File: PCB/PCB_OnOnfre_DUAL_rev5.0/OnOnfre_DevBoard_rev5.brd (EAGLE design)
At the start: 44 x 43.9 mm, 30 parts, among them J3Y S8050, J7 8p, K1 OMRON-G3MB-202P-SSR2, K2 OMRON-G3MB-202P-SSR2, U2 esp12

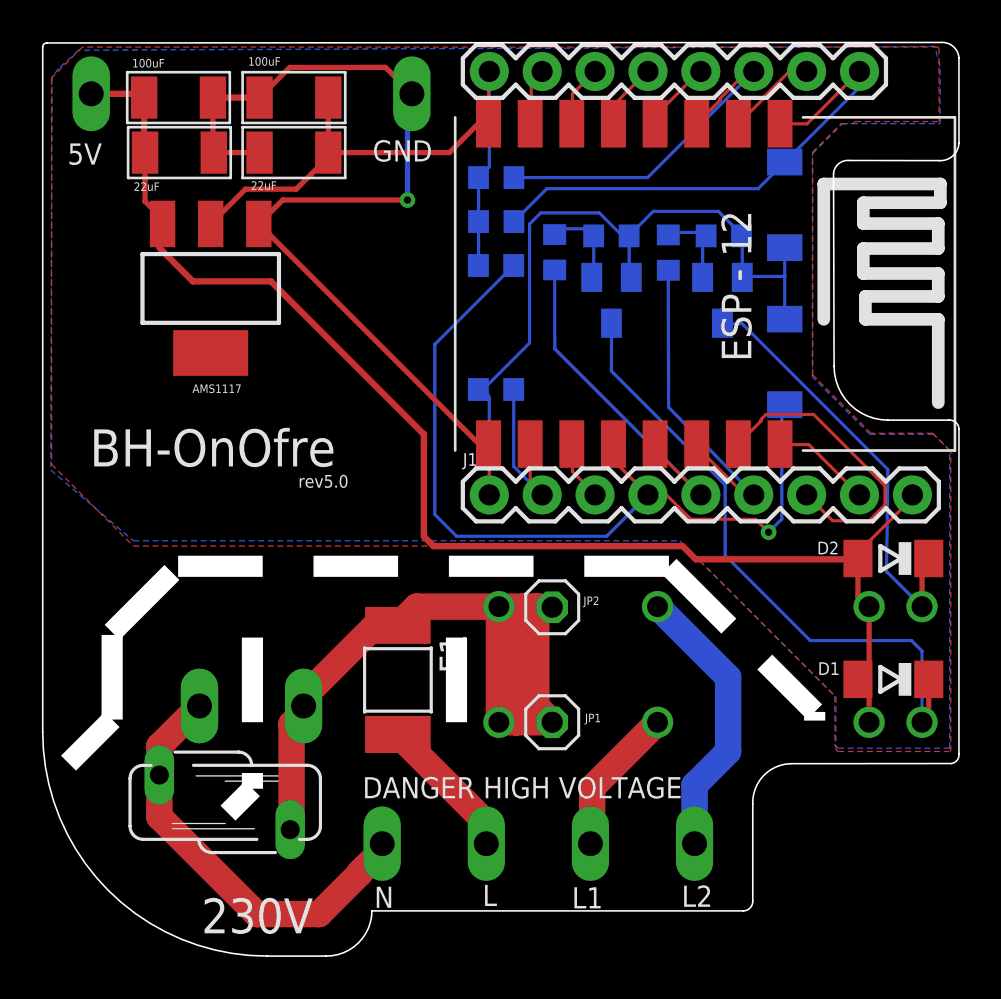
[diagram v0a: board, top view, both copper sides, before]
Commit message: rev5
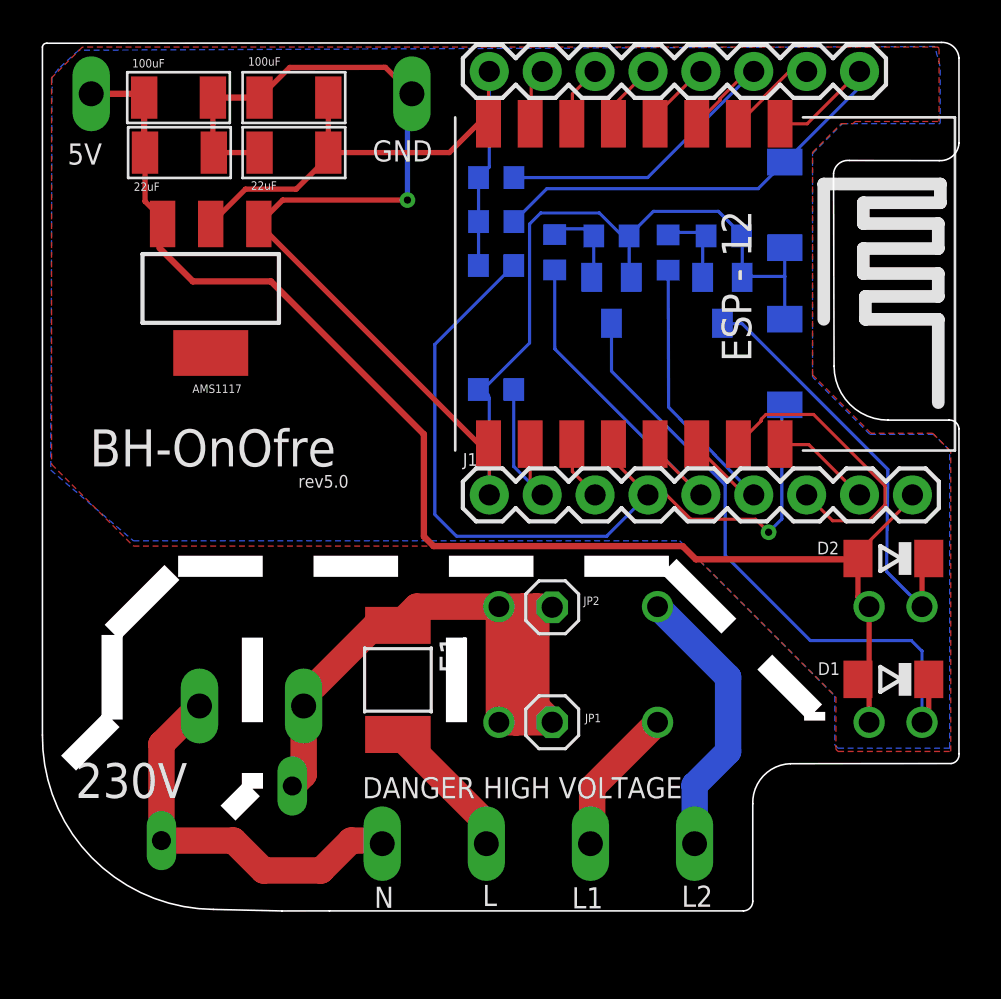
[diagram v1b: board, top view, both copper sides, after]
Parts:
- moved R5 0.54 mm to (9.56, 9.35), flipped to the bottom, turned to 270 degrees
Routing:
- net LINE_L: track 40.0 -> 37.7 mm
- net NEUTRAL_IN: track 20.1 -> 19.1 mm
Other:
- board size 44 x 43.9 mm -> 44 x 41.7 mm
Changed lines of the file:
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@@
 <grid distance="0.000123031496" unitdist="mil" unit="mil" style="lines" multiple="1" display="yes" altdistance="5" altunitdist="mil" altunit="mil"/>
 <layers>
-<layer number="1" name="Top" color="4" fill="1" visible="no" active="yes"/>
+<layer number="1" name="Top" color="4" fill="1" visible="yes" active="yes"/>
 <layer number="2" name="Route2" color="1" fill="3" visible="no" active="no"/>
 <layer number="3" name="Route3" color="4" fill="3" visible="no" active="no"/>
@@
 <layer number="25" name="tNames" color="7" fill="1" visible="yes" active="yes"/>
 <layer number="26" name="bNames" color="7" fill="1" visible="yes" active="yes"/>
-<layer number="27" name="tValues" color="7" fill="1" visible="yes" active="yes"/>
-<layer number="28" name="bValues" color="7" fill="1" visible="yes" active="yes"/>
+<layer number="27" name="tValues" color="7" fill="1" visible="no" active="yes"/>
+<layer number="28" name="bValues" color="7" fill="1" visible="no" active="yes"/>
 <layer number="29" name="tStop" color="7" fill="3" visible="no" active="yes"/>
 <layer number="30" name="bStop" color="7" fill="6" visible="no" active="yes"/>
@@
 <layer number="42" name="bRestrict" color="1" fill="10" visible="yes" active="yes"/>
 <layer number="43" name="vRestrict" color="2" fill="10" visible="no" active="yes"/>
-<layer number="44" name="Drills" color="7" fill="1" visible="yes" active="yes"/>
-<layer number="45" name="Holes" color="7" fill="1" visible="yes" active="yes"/>
-<layer number="46" name="Milling" color="3" fill="1" visible="yes" active="yes"/>
+<layer number="44" name="Drills" color="7" fill="1" visible="no" active="yes"/>
+<layer number="45" name="Holes" color="7" fill="1" visible="no" active="yes"/>
+<layer number="46" name="Milling" color="3" fill="1" visible="no" active="yes"/>
 <layer number="47" name="Measures" color="7" fill="1" visible="no" active="yes"/>
 <layer number="48" name="Document" color="7" fill="1" visible="no" active="yes"/>
@@
 <text x="33.608865625" y="25.98010625" size="0.6096" layer="26" font="vector" ratio="13" rot="MR45">L1</text>
 <text x="36.1006125" y="26.021965625" size="0.6096" layer="26" font="vector" ratio="13" rot="MR45">L2</text>
-<text x="8.320915625" y="3.579975" size="1.6764" layer="25" font="vector" ratio="13">230V</text>
+<text x="2.2720875" y="10.07901875" size="1.6764" layer="25" font="vector" ratio="13">230V</text>
 <text x="27.607209375" y="5.793196875" size="1.016" layer="25" font="vector" ratio="13" rot="R180">L1</text>
 <text x="12.972021875" y="24.981884375" size="0.6096" layer="25">rev5.0</text>
 <text x="12.192" y="12.446" size="0.4064" layer="26" rot="MR0">HLK-PM01</text>
-<wire x1="0.6984" y1="46.1592125" x2="0.6984" y2="13.243003125" width="0.0762" layer="20"/>
-<wire x1="0.6984" y1="13.243003125" x2="11.463928125" y2="2.487625" width="0.0762" layer="20" curve="90"/>
-<wire x1="11.463928125" y1="2.487625" x2="14.302721875" y2="2.487625" width="0.0762" layer="20"/>
-<wire x1="14.302721875" y1="2.487625" x2="16.511228125" y2="4.65789375" width="0.0762" layer="20" curve="90"/>
-<wire x1="16.511228125" y1="4.65789375" x2="34.35341875" y2="4.65789375" width="0.0762" layer="20"/>
+<wire x1="0.68574375" y1="46.14655625" x2="0.68574375" y2="13.103775" width="0.0762" layer="20"/>
+<wire x1="0.68574375" y1="13.103775" x2="8.892471875" y2="4.72859375" width="0.0762" layer="20" curve="90"/>
+<wire x1="8.892471875" y1="4.72859375" x2="12.19380625" y2="4.654959375" width="0.0762" layer="20"/>
+<wire x1="12.19380625" y1="4.654959375" x2="14.468953125" y2="4.657896875" width="0.0762" layer="20"/>
+<wire x1="14.468953125" y1="4.657896875" x2="34.35341875" y2="4.65789375" width="0.0762" layer="20"/>
 <wire x1="34.35341875" y1="4.65789375" x2="34.797584375" y2="5.127553125" width="0.0762" layer="20" curve="90"/>
 <wire x1="34.797584375" y1="5.127553125" x2="34.797584375" y2="9.799765625" width="0.0762" layer="20"/>
@@
 <wire x1="44.701484375" y1="41.521734375" x2="44.701475" y2="45.615690625" width="0.0762" layer="20"/>
 <wire x1="44.701475" y1="45.615690625" x2="43.848703125" y2="46.364371875" width="0.0762" layer="20" curve="90"/>
-<wire x1="43.848703125" y1="46.364371875" x2="0.916678125" y2="46.33838125" width="0.0762" layer="20"/>
-<wire x1="0.916678125" y1="46.33838125" x2="0.6984" y2="46.1592125" width="0.0762" layer="20" curve="90"/>
+<wire x1="43.848703125" y1="46.364371875" x2="0.904021875" y2="46.325725" width="0.0762" layer="20"/>
+<wire x1="0.904021875" y1="46.325725" x2="0.68574375" y2="46.14655625" width="0.0762" layer="20" curve="90"/>
 <wire x1="1.939596875" y1="11.7530875" x2="4.032321875" y2="13.8458125" width="1.016" layer="46" style="shortdash"/>
 <wire x1="4.032321875" y1="13.8458125" x2="4.032321875" y2="18.038434375" width="1.016" layer="46" style="shortdash"/>
@@
 <attribute name="OC_NEWARK" value="78R5551" x="17.757009375" y="15.7501125" size="1.778" layer="27" rot="R270" display="off"/>
 </element>
-<element name="R5" library="VARISTORESBH" package="S07K230" value="S07K230" x="9.46375625" y="9.87105625" smashed="yes" rot="R90">
-<attribute name="VALUE" x="13.52775625" y="13.93505625" size="1.27" layer="27" ratio="10" rot="R180"/>
+<element name="R5" library="VARISTORESBH" package="S07K230" value="S07K230" x="9.563103125" y="9.34500625" smashed="yes" rot="MR270">
+<attribute name="VALUE" x="13.627103125" y="5.28100625" size="1.27" layer="28" ratio="10" rot="MR0"/>
 </element>
 </elements>
@@
 <contactref element="X1" pad="1"/>
 <contactref element="R5" pad="2"/>
-<wire x1="15.931246875" y1="6.462596875" x2="13.971084375" y2="4.502434375" width="1.27" layer="1"/>
-<wire x1="17.003271875" y1="7.581321875" x2="15.931246875" y2="6.509296875" width="1.27" layer="1"/>
-<wire x1="15.931246875" y1="6.509296875" x2="15.931246875" y2="6.462596875" width="1.27" layer="1"/>
-<wire x1="13.971084375" y1="4.502434375" x2="10.976684375" y2="4.502434375" width="1.27" layer="1"/>
-<wire x1="6.300946875" y1="9.178171875" x2="6.300946875" y2="11.182271875" width="1.27" layer="1"/>
-<wire x1="10.976684375" y1="4.502434375" x2="6.300946875" y2="9.178171875" width="1.27" layer="1"/>
-<wire x1="8.22843125" y1="14.497953125" x2="6.300946875" y2="12.57046875" width="1.27" layer="1"/>
-<wire x1="6.300946875" y1="12.57046875" x2="6.300946875" y2="11.182271875" width="1.27" layer="1"/>
-<wire x1="17.003271875" y1="7.581321875" x2="17.003271875" y2="7.885928125" width="0" layer="19" extent="1-1"/>
+<wire x1="8.22843125" y1="14.497953125" x2="6.40029375" y2="12.669815625" width="1.27" layer="1"/>
+<wire x1="6.40029375" y1="12.669815625" x2="6.40029375" y2="8.033790625" width="1.27" layer="1"/>
+<wire x1="16.855409375" y1="8.033790625" x2="17.003271875" y2="7.885928125" width="1.27" layer="1"/>
+<wire x1="6.40029375" y1="8.033790625" x2="9.863371875" y2="8.033790625" width="1.27" layer="1"/>
+<wire x1="9.863371875" y1="8.033790625" x2="11.29835" y2="6.5988125" width="1.27" layer="1"/>
+<wire x1="11.29835" y1="6.5988125" x2="14.0704375" y2="6.5988125" width="1.27" layer="1"/>
+<wire x1="14.0704375" y1="6.5988125" x2="15.505415625" y2="8.033790625" width="1.27" layer="1"/>
+<wire x1="15.505415625" y1="8.033790625" x2="16.855409375" y2="8.033790625" width="1.27" layer="1"/>
 </signal>
 <signal name="N$9">
@@
 <wire x1="18.655975" y1="19.269078125" x2="22.606" y2="19.269078125" width="1.27" layer="1"/>
 <contactref element="U$1" pad="1"/>
-<wire x1="13.22843125" y1="14.497953125" x2="13.418453125" y2="14.687975" width="1.27" layer="1"/>
 <wire x1="13.418453125" y1="14.687975" x2="13.418453125" y2="15.111559375" width="1.27" layer="1"/>
 <wire x1="13.418453125" y1="15.111559375" x2="16.67700625" y2="18.3701125" width="1.27" layer="1"/>
 <wire x1="16.67700625" y1="18.3701125" x2="17.757009375" y2="18.3701125" width="1.27" layer="1"/>
 <contactref element="R5" pad="1"/>
-<wire x1="12.6492" y1="13.6398" x2="12.6492" y2="8.6106" width="1.27" layer="1"/>
-<wire x1="12.954" y1="13.9446" x2="12.6492" y2="13.6398" width="1.27" layer="1"/>
-<wire x1="12.6492" y1="8.6106" x2="12.58504375" y2="8.559840625" width="1.27" layer="1"/>
-<wire x1="12.954" y1="13.9446" x2="13.22843125" y2="14.497953125" width="1.27" layer="1"/>
+<wire x1="13.22843125" y1="14.497953125" x2="13.22843125" y2="11.2002625" width="1.27" layer="1"/>
+<wire x1="13.22843125" y1="11.2002625" x2="12.684390625" y2="10.656221875" width="1.27" layer="1"/>
+<wire x1="13.22843125" y1="14.497953125" x2="13.418453125" y2="14.687975" width="0" layer="19" extent="1-1"/>
 </signal>
 <signal name="N$2">
